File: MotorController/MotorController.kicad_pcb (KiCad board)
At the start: 2 copper layers, 49 x 26 mm, 2 parts, among them U1 TMC2209_SILENTSTEPSTICK

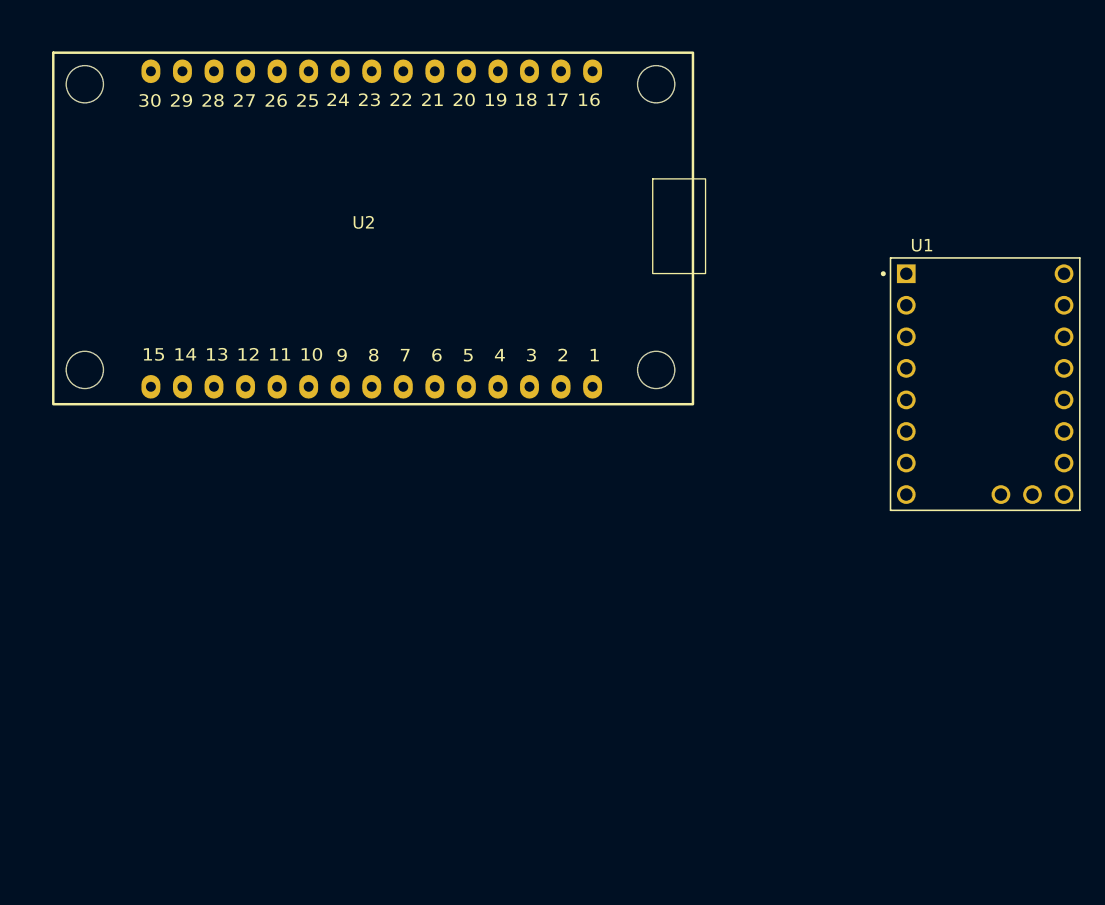
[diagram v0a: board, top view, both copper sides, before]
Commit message: 2 Driver Design Done
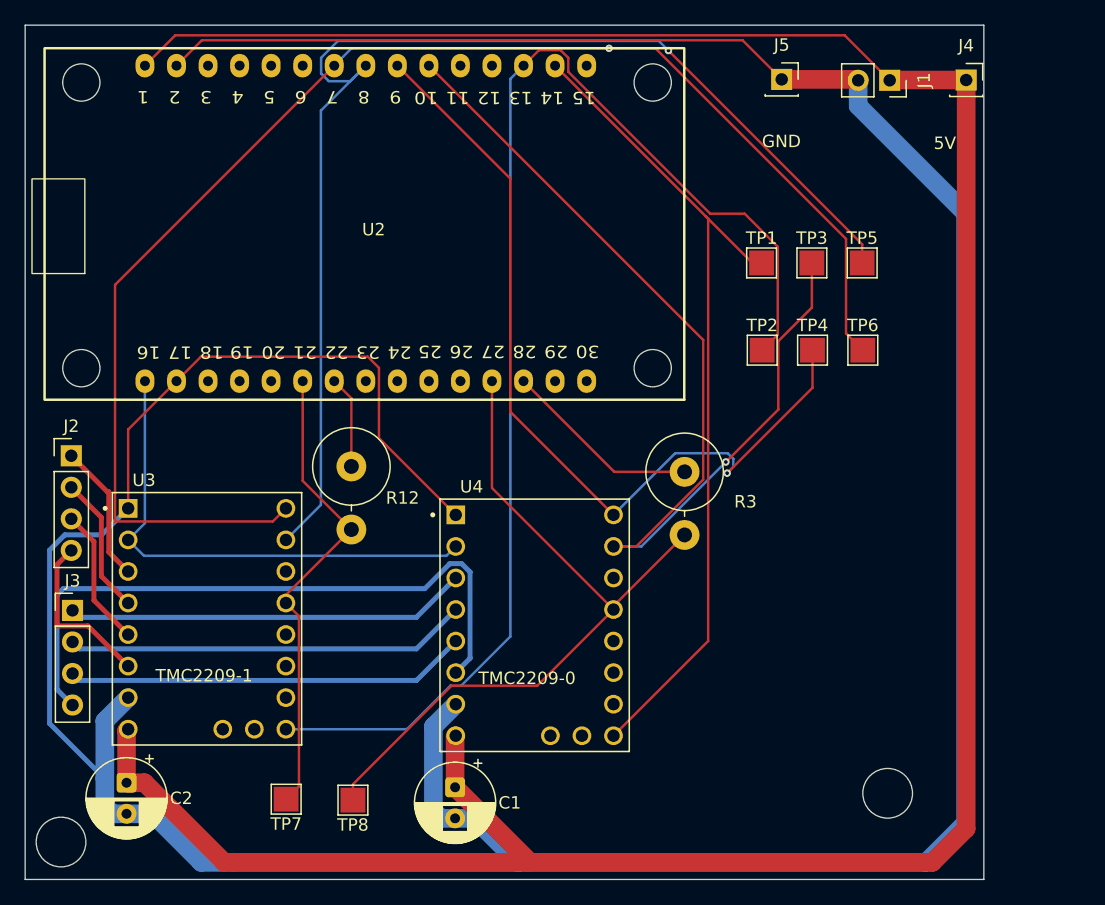
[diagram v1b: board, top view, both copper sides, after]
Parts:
- removed U1: TMC2209_SILENTSTEPSTICK, TMC2209_SILENTSTEPSTICK:MODULE_TMC2209_SILENTSTEPSTICK
- added C1: 470u, Capacitor_THT:CP_Radial_D6.3mm_P2.50mm, F.Cu at (66.7, 87.3)
- added C2: 470u, Capacitor_THT:CP_Radial_D6.3mm_P2.50mm, F.Cu at (40.2, 87.0)
- added J1: Conn_01x02_Pin, Connector_PinSocket_2.54mm:PinSocket_1x02_P2.54mm_Vertical, F.Cu at (101.7, 30.4)
- added J2: Conn_01x04_Pin, Connector_PinHeader_2.54mm:PinHeader_1x04_P2.54mm_Vertical, F.Cu at (35.8, 60.6)
- added J3: Conn_01x04_Pin, Connector_PinHeader_2.54mm:PinHeader_1x04_P2.54mm_Vertical, F.Cu at (35.9, 73.1)
- added J4: Conn_01x01_Pin, Connector_PinSocket_2.54mm:PinSocket_1x01_P2.54mm_Vertical, F.Cu at (107.8, 30.4)
- added J5: Conn_01x01_Pin, Connector_PinSocket_2.54mm:PinSocket_1x01_P2.54mm_Vertical, F.Cu at (93.0, 30.3)
- added R12: 1K, Resistor_THT:R_Axial_DIN0617_L17.0mm_D6.0mm_P5.08mm_Vertical, F.Cu at (58.4, 61.5)
- added R3: 1K, Resistor_THT:R_Axial_DIN0617_L17.0mm_D6.0mm_P5.08mm_Vertical, F.Cu at (85.2, 61.9)
- added TP1: EN1, TestPoint:TestPoint_Pad_2.0x2.0mm, F.Cu at (91.4, 45.1)
- added TP2: EN2, TestPoint:TestPoint_Pad_2.0x2.0mm, F.Cu at (91.4, 52.1)
- added TP3: STEP1, TestPoint:TestPoint_Pad_2.0x2.0mm, F.Cu at (95.4, 45.1)
- added TP4: DIR1, TestPoint:TestPoint_Pad_2.0x2.0mm, F.Cu at (95.5, 52.1)
- added TP5: STEP2, TestPoint:TestPoint_Pad_2.0x2.0mm, F.Cu at (99.5, 45.1)
- added TP6: DIR2, TestPoint:TestPoint_Pad_2.0x2.0mm, F.Cu at (99.5, 52.1)
- added TP7: UART2, TestPoint:TestPoint_Pad_2.0x2.0mm, F.Cu at (53.1, 88.3)
- added TP8: UART1, TestPoint:TestPoint_Pad_2.0x2.0mm, F.Cu at (58.5, 88.3)
- added U3: TMC2209_SILENTSTEPSTICK, TMC2209_SILENTSTEPSTICK:MODULE_TMC2209_SILENTSTEPSTICK, F.Cu at (46.7, 73.8)
- added U4: TMC2209_SILENTSTEPSTICK, TMC2209_SILENTSTEPSTICK:MODULE_TMC2209_SILENTSTEPSTICK, F.Cu at (73.1, 74.3)
- turned U2 to 180 degrees
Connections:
- U2 pad 1: unconnected-(U2-VIN-Pad1) -> +5V
- U2 pad 10: unconnected-(U2-GPIO32-Pad10) -> /STEP1
- U2 pad 13: unconnected-(U2-GPIO39-Pad13) -> /EN2
- U2 pad 14: unconnected-(U2-GPIO36-Pad14) -> /EN1
- U2 pad 16: unconnected-(U2-3.3v-Pad16) -> +3V3
- U2 pad 17: unconnected-(U2-GND-Pad17) -> GND
- U2 pad 2: unconnected-(U2-GND-Pad2) -> GND
- U2 pad 21: unconnected-(U2-GPIO16-Pad21) -> /UART2
- U2 pad 22: unconnected-(U2-GPIO17-Pad22) -> Net-(U2-GPIO17)
- U2 pad 27: unconnected-(U2-GPIO3-Pad27) -> /UART1
- U2 pad 28: unconnected-(U2-GPIO1-Pad28) -> Net-(U2-GPIO1)
- U2 pad 7: unconnected-(U2-GPIO26-Pad7) -> /DIR2
- U2 pad 8: unconnected-(U2-GPIO25-Pad8) -> /STEP2
- U2 pad 9: unconnected-(U2-GPIO33-Pad9) -> /DIR1
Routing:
- net GND: track 0.00 -> 292.0 mm
- net +5V: track 0.00 -> 217.3 mm
- net /DIR2: track 0.00 -> 115.8 mm, vias 0 -> 1
- net /EN2: track 0.00 -> 104.6 mm
- net /STEP2: track 0.00 -> 98.9 mm, vias 0 -> 1
- net /STEP1: track 0.00 -> 82.7 mm, vias 0 -> 1
- net /DIR1: track 0.00 -> 69.4 mm, vias 0 -> 1
- net /EN1: track 0.00 -> 68.3 mm
- net /UART1: track 0.00 -> 58.9 mm
- net Net-(J3-Pin_4): track 0.00 -> 52.5 mm
- net +3V3: track 0.00 -> 40.6 mm
- net /UART2: track 0.00 -> 38.3 mm
- net Net-(J3-Pin_2): track 0.00 -> 32.4 mm
- net Net-(J3-Pin_3): track 0.00 -> 32.4 mm
- net Net-(J3-Pin_1): track 0.00 -> 32.4 mm
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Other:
- board size 49 x 26 mm -> 77.2 x 68.8 mm
- board text added: "5V"
- board text added: "GND"
- board text added: "TMC2209-0"
- board text added: "TMC2209-1"
